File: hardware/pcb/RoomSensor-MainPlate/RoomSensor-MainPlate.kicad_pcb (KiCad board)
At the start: 4 copper layers, 31 x 54 mm, 9 parts, among them J1 B2B_Connector

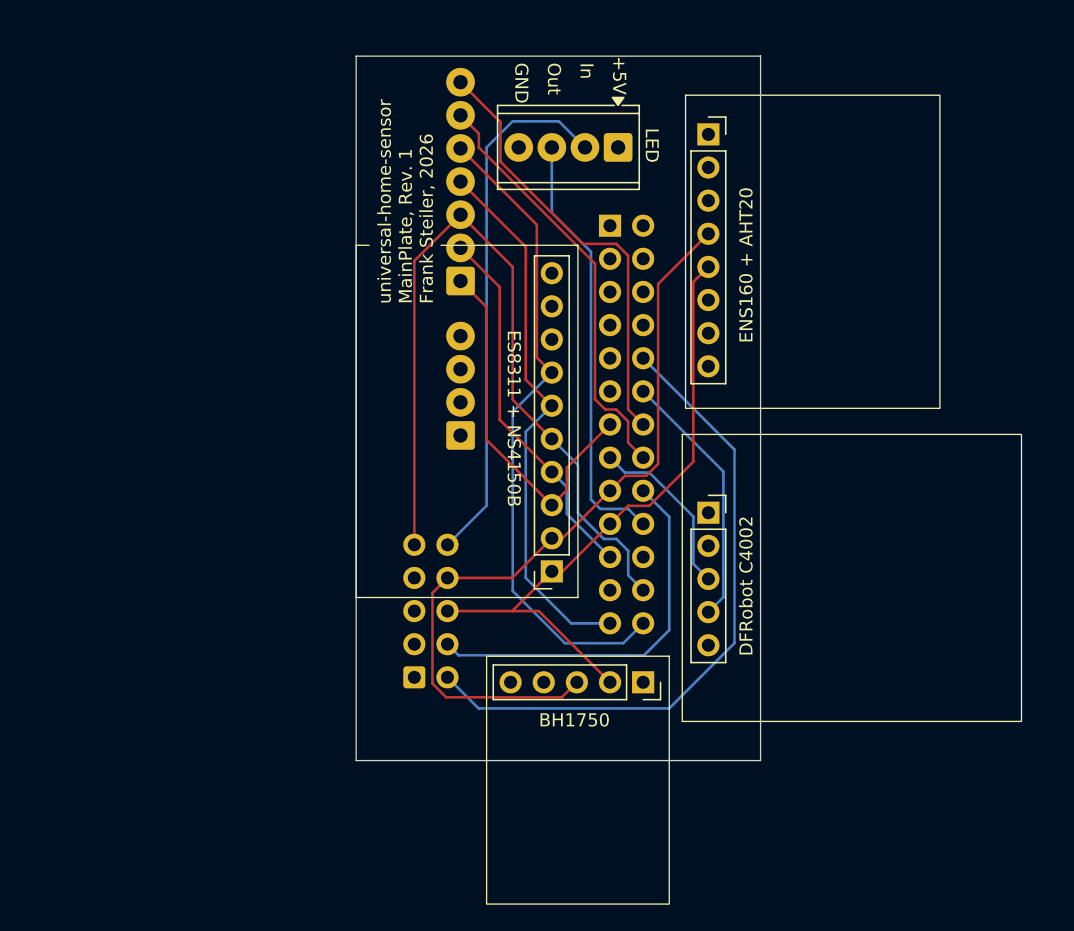
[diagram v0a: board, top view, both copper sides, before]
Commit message: Updated PCB to Rev 2 and 3
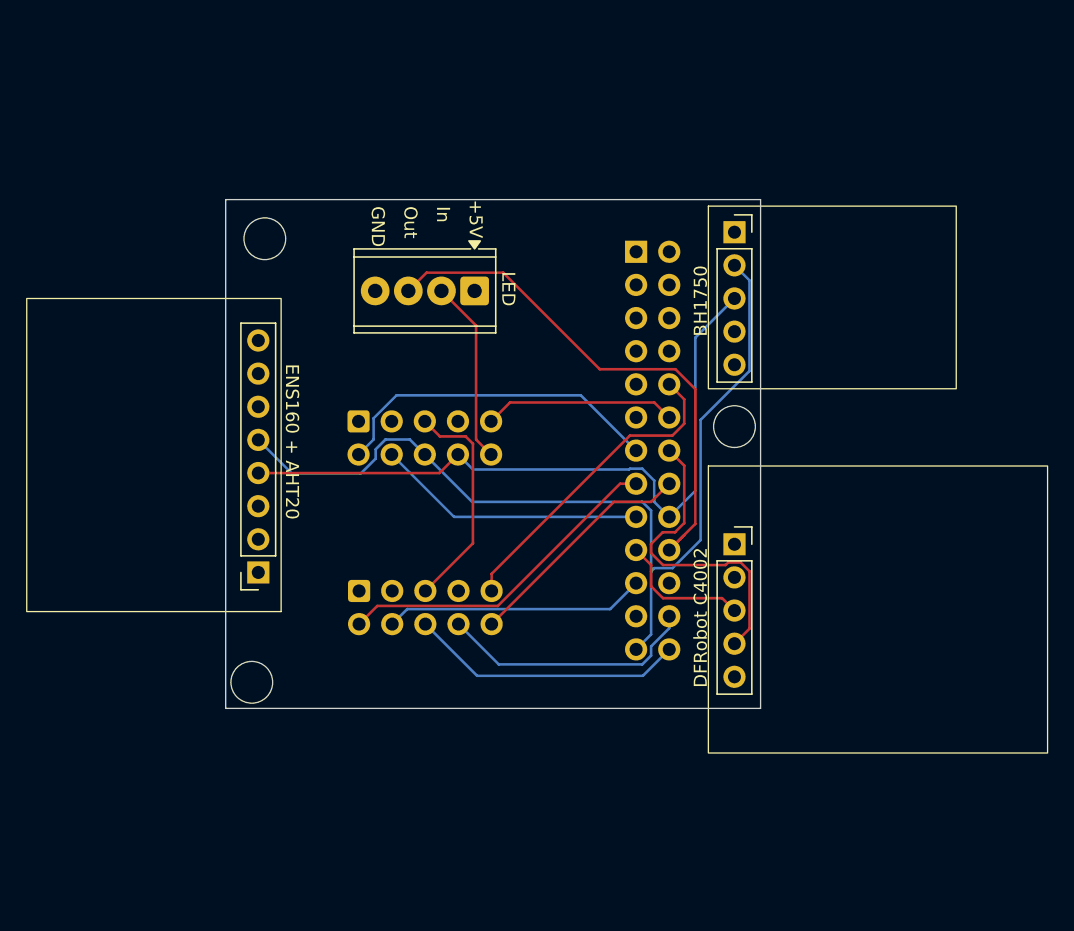
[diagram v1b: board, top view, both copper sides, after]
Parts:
- removed A1: ES8311 + NS4150B, room-sensor:ES8311 + NS4150B Connector
- removed C2: Power, TerminalBlock_Phoenix:TerminalBlock_Phoenix_MPT-0,5-4-2.54_1x04_P2.54mm_Horizontal
- removed C3: GPIO, TerminalBlock_Phoenix:TerminalBlock_Phoenix_MPT-0,5-7-2.54_1x07_P2.54mm_Horizontal
- added J2: GPIO, Connector_IDC:IDC-Header_2x05_P2.54mm_Vertical, B.Cu at (70.2, 83.0)
- moved S3 48.1 mm to (62.5, 81.6), turned to 180 degrees
- moved S2 35.2 mm to (99.0, 55.5), turned to 0 degrees
- moved J1 20.1 mm to (70.2, 70.0), turned to -90 degrees
- moved C1 15.6 mm to (79.1, 60.0)
- moved S1 3.14 mm to (99.0, 79.4)
- moved E1 2.83 mm to (91.5, 57.0)
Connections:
- E1 pad 10: /E_RX -> Net-(E1-GPI39)
- E1 pad 12: /M_RX -> Net-(E1-GPI36)
- E1 pad 13: /A_MCLK -> /E_RX
- E1 pad 14: Net-(C3-GPI35) -> /M_RX
- E1 pad 15: /M_TX -> Net-(E1-GPIO2)
- E1 pad 17: /SCL -> /E_TX
- E1 pad 18: /E_TX -> /SCL
- E1 pad 19: /SDA -> /M_TX
- E1 pad 21: /A_BCLK -> Net-(E1-GPIO5)
- E1 pad 24: /A_DI -> Net-(E1-GPIO15)
- E1 pad 25: /A_LRCLK -> /SDA
- E1 pad 26: /A_DO -> Net-(E1-GPIO14)
- J1 pad 9: /A_DI -> Net-(E1-GPI36)
- S2 pad 5: /+5V -> /+3.3V
- S3 pad 1: /+5V -> unconnected-(S3-Vin-Pad1)
- S3 pad 2: unconnected-(S3-3V3-Pad2) -> /+3.3V
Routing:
- net /A_DI: track 61.9 -> 0.00 mm
- net /A_DO: track 50.3 -> 0.00 mm
- net /A_LRCLK: track 42.0 -> 0.00 mm
- net Net-(C3-GPI35): track 33.6 -> 0.00 mm
- net /A_BCLK: track 28.4 -> 0.00 mm
- net /A_MCLK: track 28.1 -> 0.00 mm
- net Net-(C1-DIn): track 40.9 -> 14.1 mm
- net Net-(E1-GPIO2): track 0.00 -> 25.7 mm
- net /SDA: track 49.3 -> 73.9 mm
- net Net-(E1-GPI39): track 0.00 -> 24.3 mm
- net /E_RX: track 49.8 -> 25.9 mm
- net /+3.3V: track 36.3 -> 57.9 mm
- net Net-(E1-GPIO14): track 0.00 -> 21.2 mm
- net Net-(E1-GPIO5): track 0.00 -> 20.0 mm
- net Net-(E1-GPIO15): track 0.00 -> 19.9 mm
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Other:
- board size 31 x 54 mm -> 41 x 39 mm
- board text added: "+12/24V"
- board text added: "+3.3V"
- board text added: "+5V"
- board text added: "GND"
- board text added: "GPI34"
- board text added: "GPI39"
- board text added: "GPIO14"
- board text added: "GPIO15"
- board text added: "GPIO2"
- board text added: "GPIO5"
- board text added: "universal-home-sensor MainPlate, Rev. 2 Frank Steiler, 2026"
- board text removed: "universal-home-sensor MainPlate, Rev. 1 Frank Steiler, 2026"
